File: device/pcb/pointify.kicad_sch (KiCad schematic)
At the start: 14 parts, among them J1 PWM, J2 JTAG, J3 USB_C, U1 XC6206P332MR, U2 STM32F070F6P6, Y1 8MHz

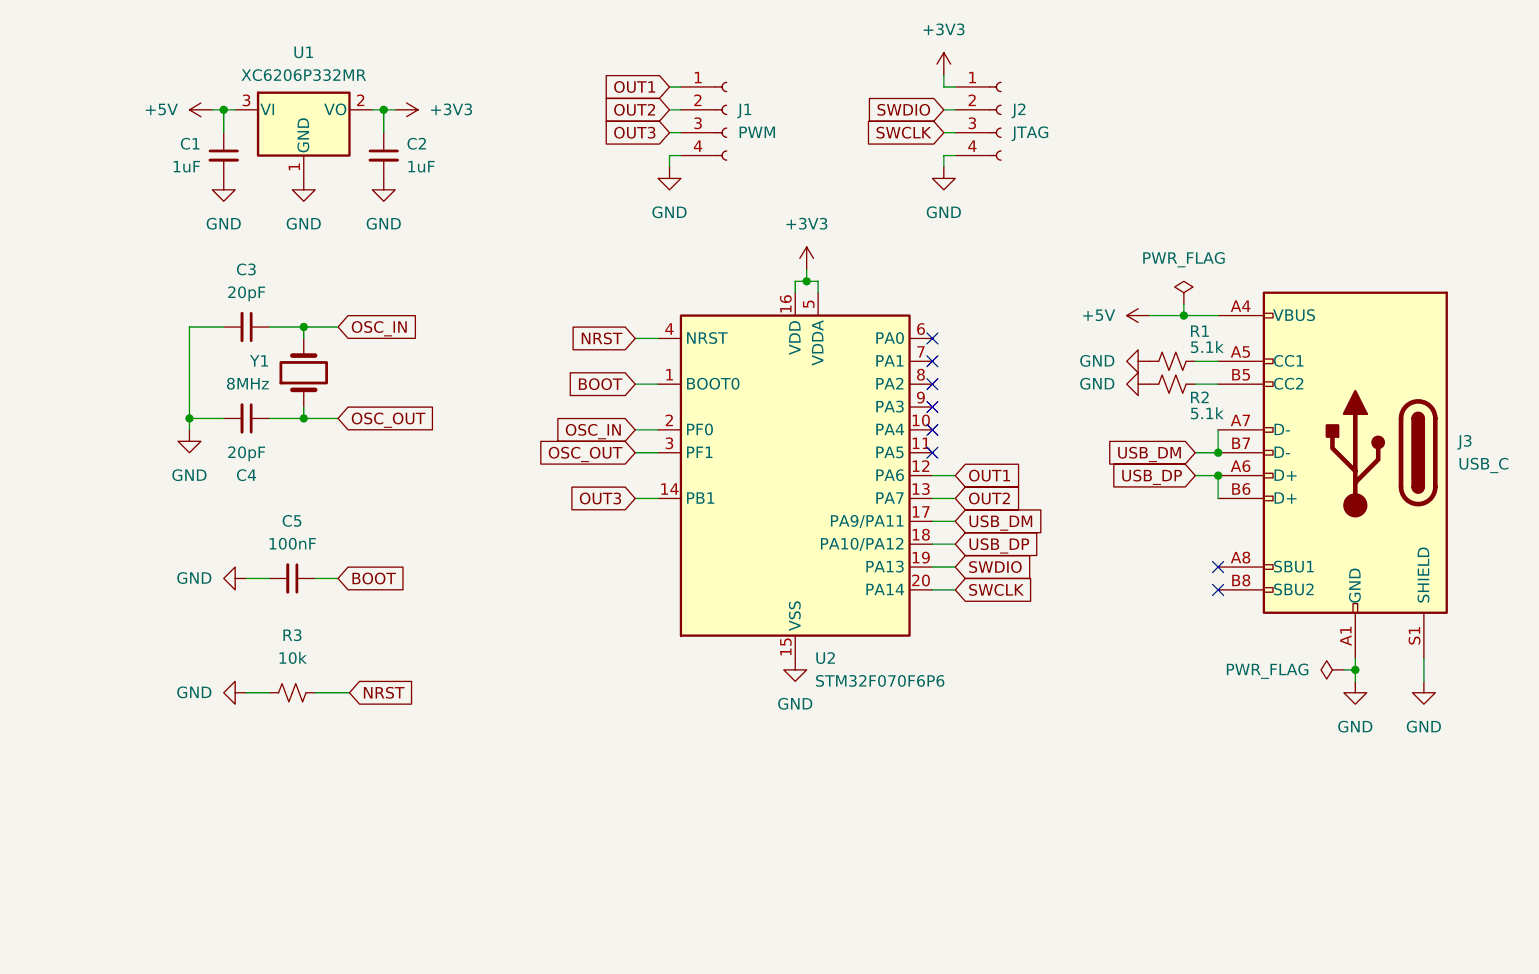
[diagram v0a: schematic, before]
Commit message: add: complete pcb artwork
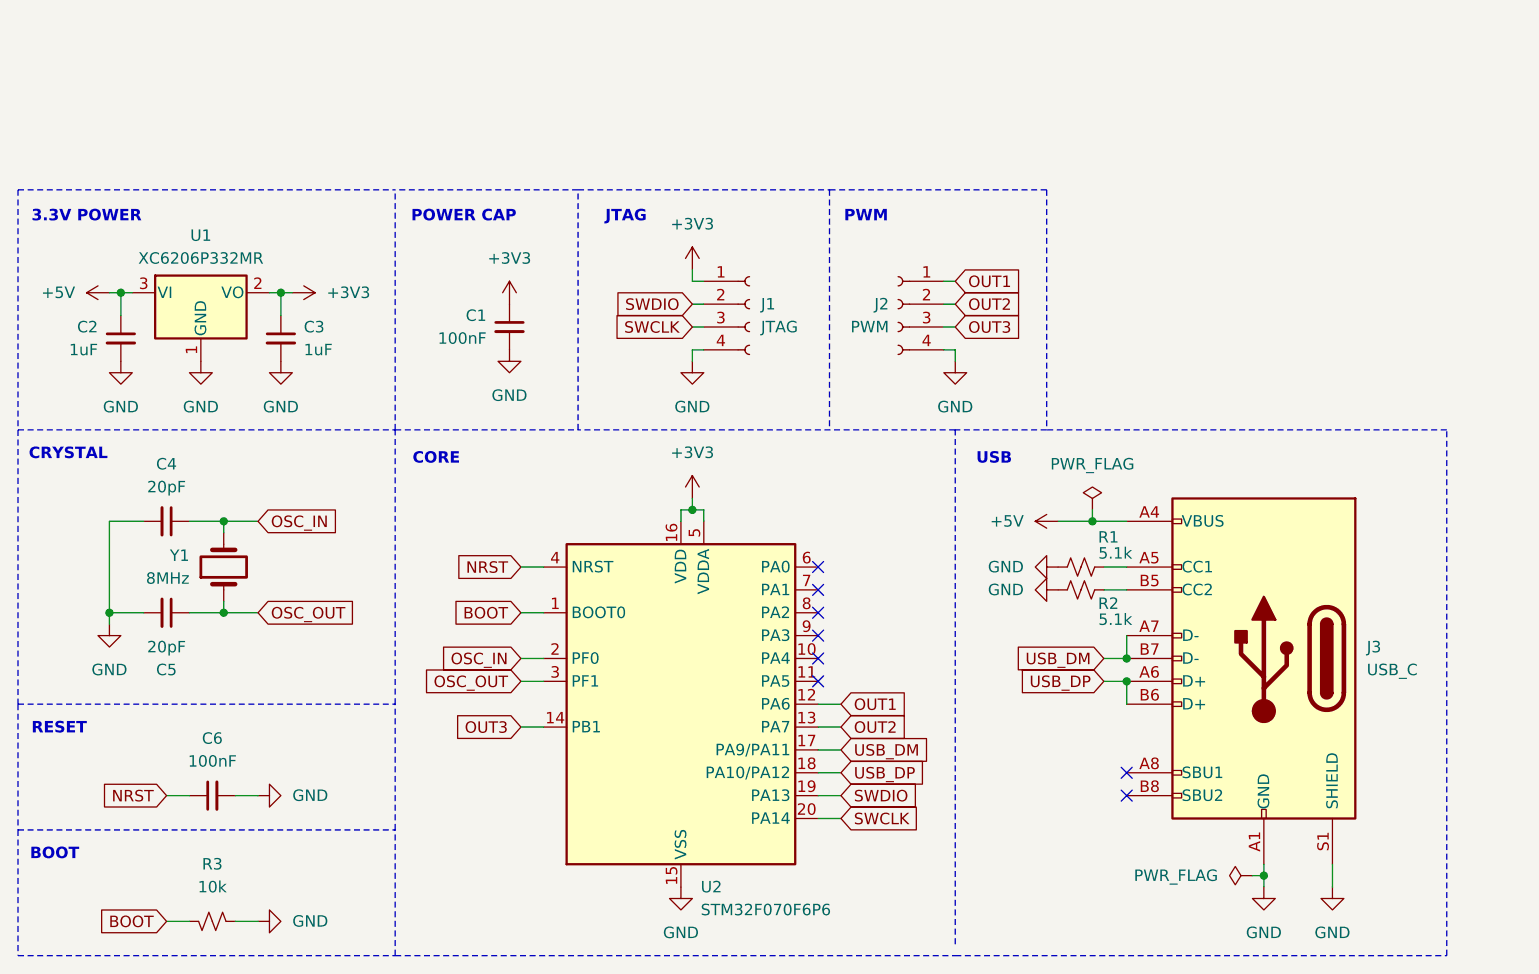
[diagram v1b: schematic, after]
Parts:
- added C1: 100nF, Capacitor_SMD:C_0603_1608Metric, symbol Device:C_Small
- C2: renamed from C1; LCSC (none) -> C15849
- C3: renamed from C2; LCSC (none) -> C15849
- C4: renamed from C3; LCSC (none) -> C1648
- C5: renamed from C4; LCSC (none) -> C1648
- C6: renamed from C5; LCSC (none) -> C14663
- J1: renamed from J2; footprint Connector_PinHeader_2.54mm:PinHeader_1x04_P2.54mm_Vertical -> Connector_PinHeader_1.27mm:PinHeader_1x04_P1.27mm_Vertical
- J3: LCSC (none) -> C165948
- R1, R2: LCSC (none) -> C23186
- R3: LCSC (none) -> C25804
- U1: LCSC (none) -> C5446
- U2: LCSC (none) -> C86951
- Y1: footprint Crystal:Crystal_SMD_HC49-SD -> Crystal:Crystal_SMD_5032-2Pin_5.0x3.2mm; LCSC (none) -> C115962
- renumbered J1 to J2
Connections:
- net +3V3: now also C1.1
- net BOOT: now also R3.2; no longer C6.1
- net GND: now also C1.2
- net NRST: now also C6.1; no longer R3.2
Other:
- note added: "3.3V POWER"
- note added: "BOOT"
- note added: "CORE"
- note added: "CRYSTAL"
- note added: "JTAG"
- note added: "POWER CAP"
- note added: "PWM"
- note added: "RESET"
- note added: "USB"
- moved on the sheet: C2, C3, C4, C5, C6, J1, J2, J3, R1, R2, R3, U1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
